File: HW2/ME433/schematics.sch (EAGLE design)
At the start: 23 parts, among them U1 PIC32MX250F128B, U2 MCP1702, Y1 8MHz

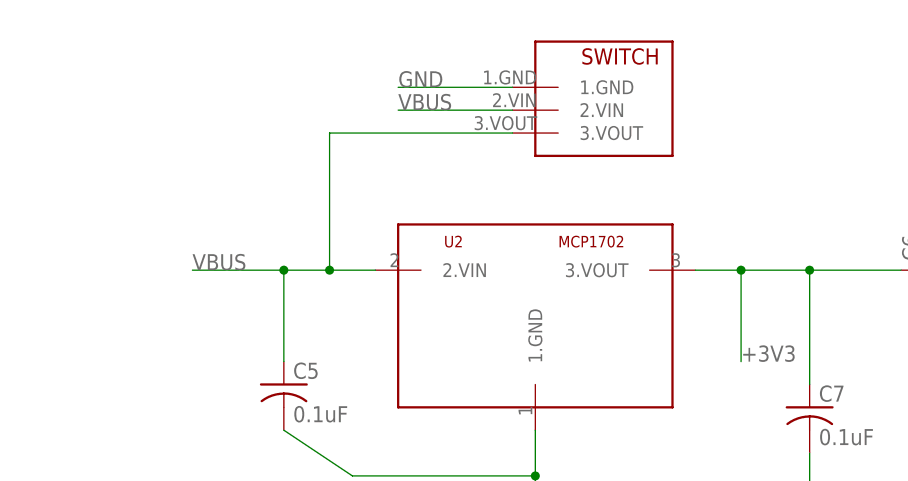
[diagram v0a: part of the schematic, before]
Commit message: Readytobecheckedbeforeorder
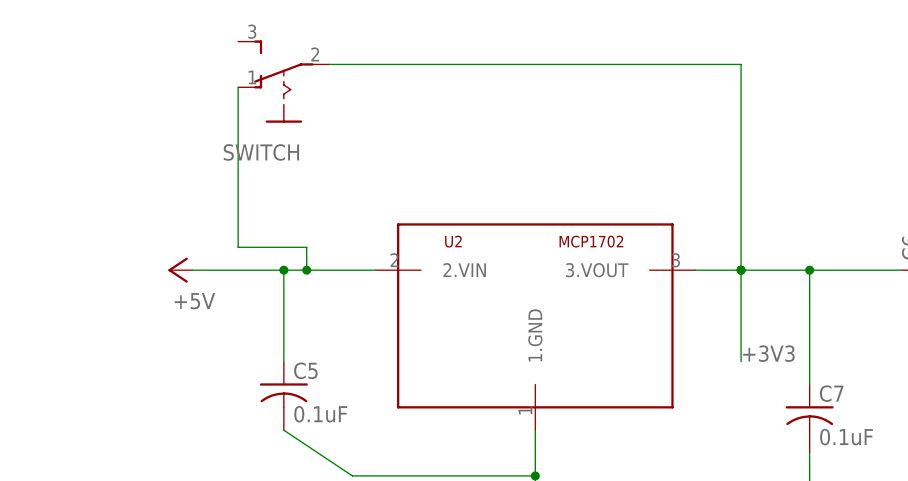
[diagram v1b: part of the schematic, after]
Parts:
- SWITCH: device libraries:SWITCH -> libraries:255SB
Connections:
- net +3V3: now also SWITCH.P
- net +5V: now also C5.1, SWITCH.O, U2.2.VIN
- net GND: no longer SWITCH.1.GND
- net VBUS: no longer C5.1, SWITCH.2.VIN, SWITCH.3.VOUT, U2.2.VIN
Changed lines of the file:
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@@
 <part name="GND11" library="libraries" deviceset="GND" device=""/>
 <part name="P+1" library="libraries" deviceset="+5V" device=""/>
-<part name="SWITCH" library="libraries" deviceset="SWITCH" device=""/>
 <part name="USB" library="libraries" deviceset="USBMINI" device=""/>
+<part name="SWITCH" library="libraries" deviceset="255SB" device=""/>
+<part name="P+2" library="libraries" deviceset="+5V" device=""/>
 </parts>
 <sheets>
@@
 <instance part="GND11" gate="1" x="27.94" y="35.56" rot="R180"/>
 <instance part="P+1" gate="1" x="132.08" y="-71.12" rot="R270"/>
-<instance part="SWITCH" gate="G$1" x="66.04" y="129.54"/>
 <instance part="USB" gate="G$1" x="167.64" y="-7.62"/>
+<instance part="SWITCH" gate="1" x="35.56" y="127" rot="R90"/>
+<instance part="P+2" gate="1" x="22.86" y="106.68" rot="R90"/>
 </instances>
 <busses>
@@
 <junction x="86.36" y="106.68"/>
 <label x="86.36" y="96.52" size="1.778" layer="95"/>
+<wire x1="86.36" y1="129.54" x2="86.36" y2="106.68" width="0.1524" layer="91"/>
+<junction x="86.36" y="106.68"/>
+<pinref part="SWITCH" gate="1" pin="P"/>
+<wire x1="40.64" y1="129.54" x2="86.36" y2="129.54" width="0.1524" layer="91"/>
 </segment>
 </net>
@@
 </segment>
 <segment>
-<pinref part="SWITCH" gate="G$1" pin="1.GND"/>
-<wire x1="60.96" y1="127" x2="48.26" y2="127" width="0.1524" layer="91"/>
-<label x="48.26" y="127" size="1.778" layer="95"/>
-</segment>
-<segment>
 <pinref part="USB" gate="G$1" pin="1.GND"/>
 <wire x1="147.32" y1="2.54" x2="134.62" y2="2.54" width="0.1524" layer="91"/>
@@
 <wire x1="99.06" y1="-10.16" x2="104.14" y2="-10.16" width="0.1524" layer="91"/>
 <label x="101.6" y="-10.16" size="1.778" layer="95"/>
-</segment>
-<segment>
-<pinref part="C5" gate="G$1" pin="1"/>
-<wire x1="35.56" y1="106.68" x2="25.4" y2="106.68" width="0.1524" layer="91"/>
-<wire x1="35.56" y1="96.52" x2="35.56" y2="106.68" width="0.1524" layer="91"/>
-<label x="25.4" y="106.68" size="1.778" layer="95"/>
-<pinref part="U2" gate="G$1" pin="2.VIN"/>
-<wire x1="45.72" y1="106.68" x2="40.64" y2="106.68" width="0.1524" layer="91"/>
-<junction x="35.56" y="106.68"/>
-<pinref part="SWITCH" gate="G$1" pin="3.VOUT"/>
-<wire x1="40.64" y1="106.68" x2="35.56" y2="106.68" width="0.1524" layer="91"/>
-<wire x1="60.96" y1="121.92" x2="40.64" y2="121.92" width="0.1524" layer="91"/>
-<wire x1="40.64" y1="121.92" x2="40.64" y2="106.68" width="0.1524" layer="91"/>
-<junction x="40.64" y="106.68"/>
-</segment>
-<segment>
-<pinref part="SWITCH" gate="G$1" pin="2.VIN"/>
-<wire x1="60.96" y1="124.46" x2="48.26" y2="124.46" width="0.1524" layer="91"/>
-<label x="48.26" y="124.46" size="1.778" layer="95"/>
 </segment>
 <segment>
@@
 <pinref part="P+1" gate="1" pin="+5V"/>
 </segment>
-</net>
+<segment>
+<pinref part="C5" gate="G$1" pin="1"/>
+<wire x1="35.56" y1="106.68" x2="25.4" y2="106.68" width="0.1524" layer="91"/>
+<wire x1="35.56" y1="96.52" x2="35.56" y2="106.68" width="0.1524" layer="91"/>
+<pinref part="U2" gate="G$1" pin="2.VIN"/>
+<wire x1="45.72" y1="106.68" x2="38.1" y2="106.68" width="0.1524" layer="91"/>
+<junction x="35.56" y="106.68"/>
+<wire x1="38.1" y1="106.68" x2="35.56" y2="106.68" width="0.1524" layer="91"/>
+<pinref part="SWITCH" gate="1" pin="O"/>
+<wire x1="30.48" y1="127" x2="30.48" y2="109.22" width="0.1524" layer="91"/>
+<wire x1="30.48" y1="109.22" x2="38.1" y2="109.22" width="0.1524" layer="91"/>
+<wire x1="38.1" y1="109.22" x2="38.1" y2="106.68" width="0.1524" layer="91"/>
+<junction x="38.1" y="106.68"/>
+<pinref part="P+2" gate="1" pin="+5V"/>
+</segment>
+</net>
